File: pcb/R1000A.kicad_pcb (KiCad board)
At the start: 2 copper layers, 182 x 104 mm, 111 parts, among them J1 PCIESOCKET-X1, J10 PCIESOCKET-X1, J11 PCIESOCKET-X1, J12 PCIESOCKET-X1, J13 PCIESOCKET-X1, J14 PCIESOCKET-X1, J15 PCIESOCKET-X1, J16 PCIESOCKET-X1, J17 USB_B_RECEPTACLE, J18 USB_B_RECEPTACLE, J2 PCIESOCKET-X1, J25 SOCKET420P-02X04-CPU, J26 SOCKET508P-01X04, J27 CONN500P-01X04, J3 PCIESOCKET-X1, J4 PCIESOCKET-X1, J5 PCIESOCKET-X1, J6 PCIESOCKET-X1, J7 PCIESOCKET-X1, J8 PCIESOCKET-X1, J9 PCIESOCKET-X1, U1 LPC1769FBD100,551, U2 AP3418, U3 NX3DV221, U4 78SRH-5/2-C

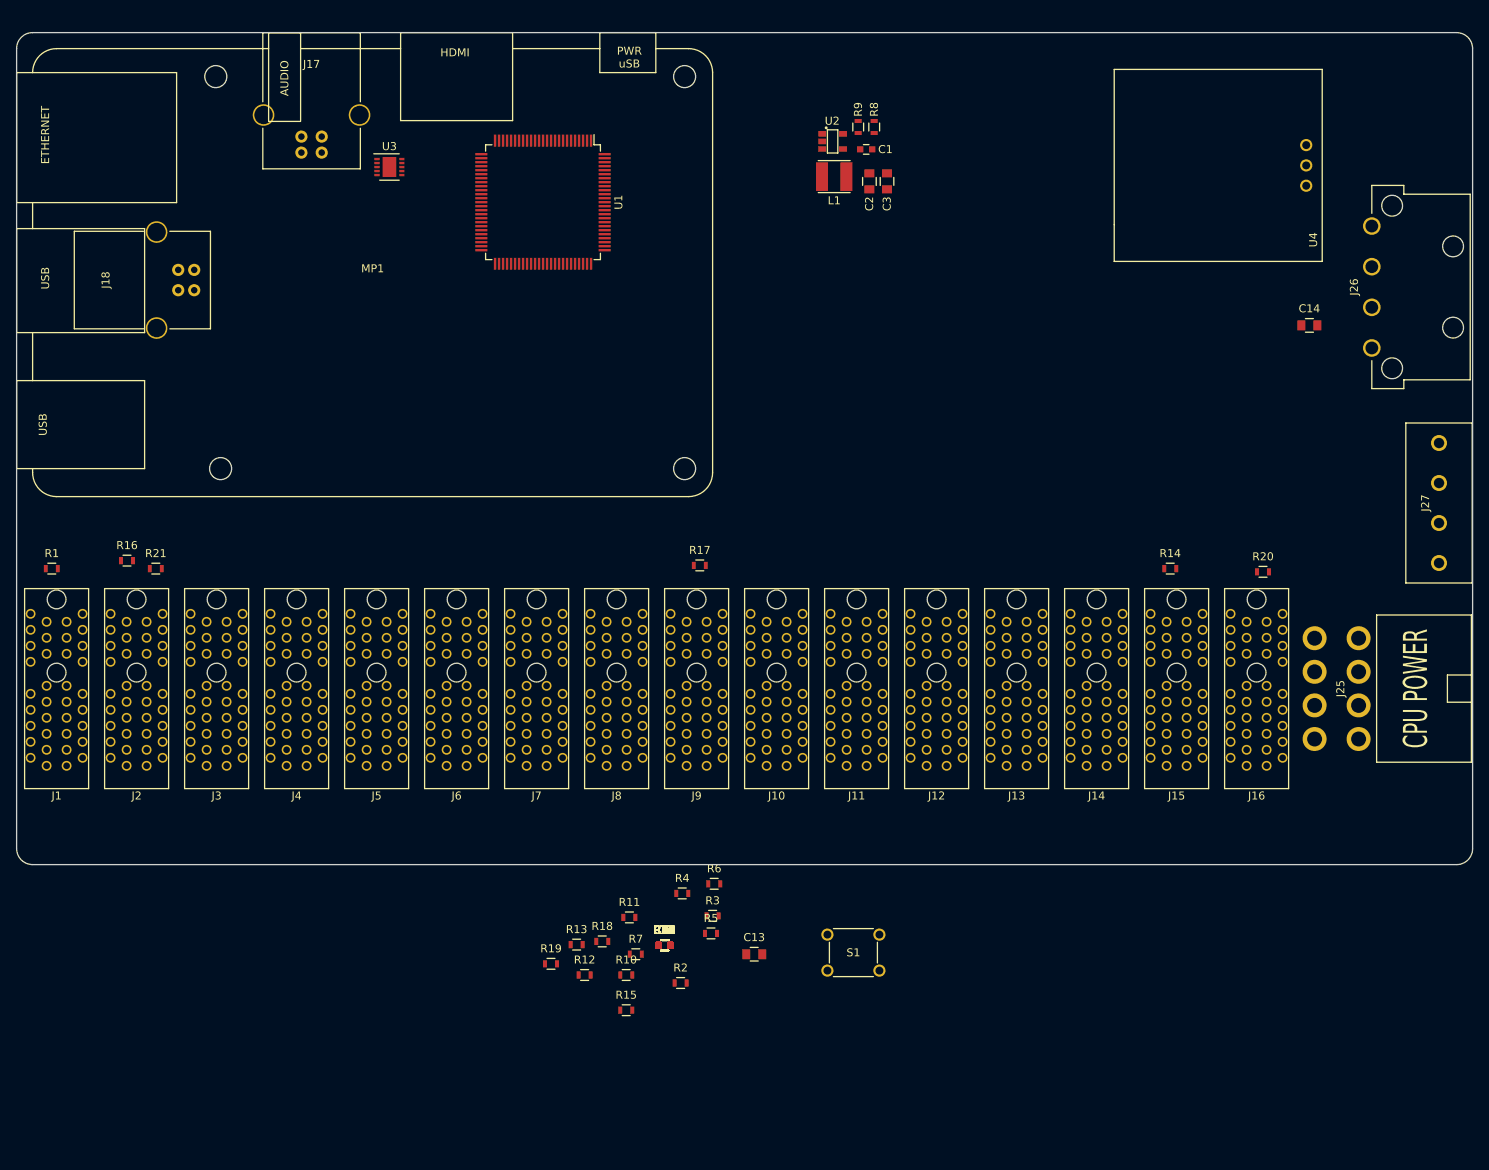
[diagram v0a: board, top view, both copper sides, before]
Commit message: layout wip
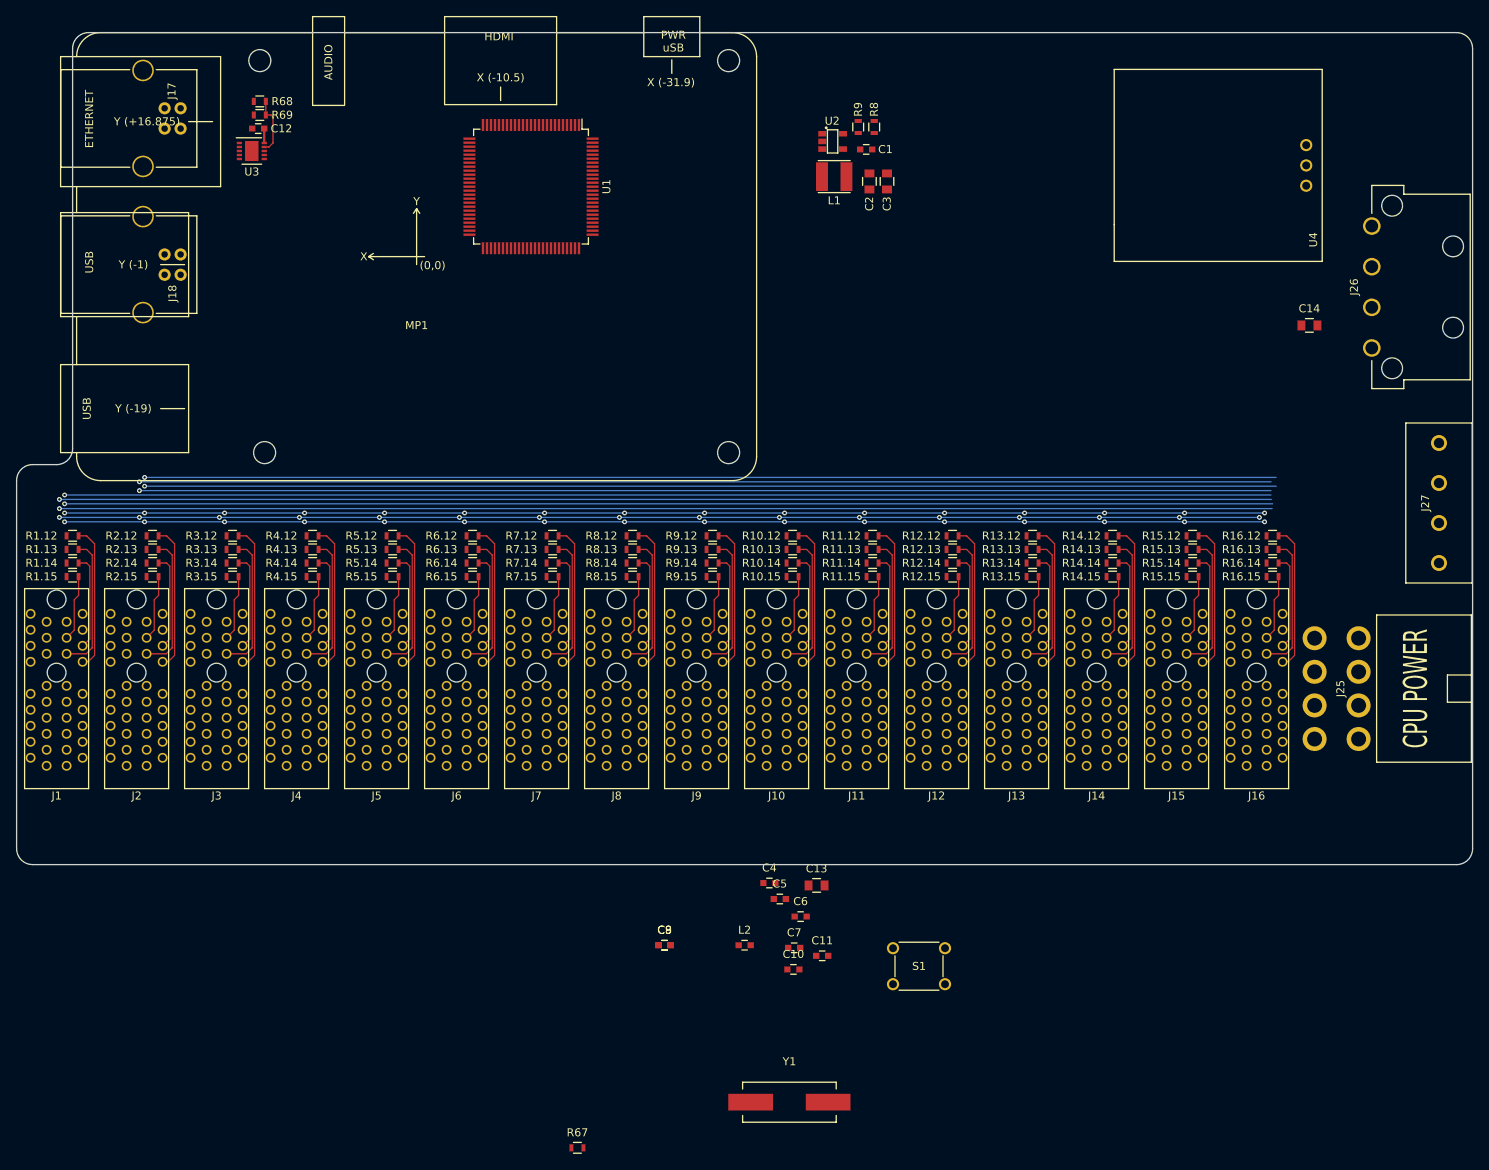
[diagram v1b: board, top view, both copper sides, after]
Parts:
- removed R1, R10, R11, R12, R13, R14, R15, R16, R17, R18, R19, R2, R20, R21, R22, R23, R24, R25, R26, R27, R28, R29, R3, R30, R31, R32, R33, R34, R35, R36, R37, R38, R39, R4, R40, R41, R42, R43, R44, R45, R46, R47, R48, R49, R5, R50, R51, R52, R53, R54, R55, R56, R57, R58, R59, R6, R60, R61, R62, R63, R64, R65, R66, R7: 10k, Resistors_SMD:R_0603
- added L2: 600Ohms, Capacitors_SMD:C_0603, F.Cu at (156.0, 152.1)
- added R1.12: 10k, Resistors_SMD:R_0603, F.Cu at (72.0, 100.9)
- added R1.13: 10k, Resistors_SMD:R_0603, F.Cu at (72.0, 102.6)
- added R1.14: 10k, Resistors_SMD:R_0603, F.Cu at (72.0, 104.3)
- added R1.15: 10k, Resistors_SMD:R_0603, F.Cu at (72.0, 106.0)
- added R10.12: 10k, Resistors_SMD:R_0603, F.Cu at (162.0, 100.9)
- added R10.13: 10k, Resistors_SMD:R_0603, F.Cu at (162.0, 102.6)
- added R10.14: 10k, Resistors_SMD:R_0603, F.Cu at (162.0, 104.3)
- added R10.15: 10k, Resistors_SMD:R_0603, F.Cu at (162.0, 106.0)
- added R11.12: 10k, Resistors_SMD:R_0603, F.Cu at (172.0, 100.9)
- added R11.13: 10k, Resistors_SMD:R_0603, F.Cu at (172.0, 102.6)
- added R11.14: 10k, Resistors_SMD:R_0603, F.Cu at (172.0, 104.3)
- added R11.15: 10k, Resistors_SMD:R_0603, F.Cu at (172.0, 106.0)
- added R12.12: 10k, Resistors_SMD:R_0603, F.Cu at (182.0, 100.9)
- added R12.13: 10k, Resistors_SMD:R_0603, F.Cu at (182.0, 102.6)
- added R12.14: 10k, Resistors_SMD:R_0603, F.Cu at (182.0, 104.3)
- added R12.15: 10k, Resistors_SMD:R_0603, F.Cu at (182.0, 106.0)
- added R13.12: 10k, Resistors_SMD:R_0603, F.Cu at (192.0, 100.9)
- added R13.13: 10k, Resistors_SMD:R_0603, F.Cu at (192.0, 102.6)
- added R13.14: 10k, Resistors_SMD:R_0603, F.Cu at (192.0, 104.3)
- added R13.15: 10k, Resistors_SMD:R_0603, F.Cu at (192.0, 106.0)
- added R14.12: 10k, Resistors_SMD:R_0603, F.Cu at (202.0, 100.9)
- added R14.13: 10k, Resistors_SMD:R_0603, F.Cu at (202.0, 102.6)
- added R14.14: 10k, Resistors_SMD:R_0603, F.Cu at (202.0, 104.3)
- added R14.15: 10k, Resistors_SMD:R_0603, F.Cu at (202.0, 106.0)
- added R15.12: 10k, Resistors_SMD:R_0603, F.Cu at (212.0, 100.9)
- added R15.13: 10k, Resistors_SMD:R_0603, F.Cu at (212.0, 102.6)
- added R15.14: 10k, Resistors_SMD:R_0603, F.Cu at (212.0, 104.3)
- added R15.15: 10k, Resistors_SMD:R_0603, F.Cu at (212.0, 106.0)
- added R16.12: 10k, Resistors_SMD:R_0603, F.Cu at (222.0, 100.9)
- added R16.13: 10k, Resistors_SMD:R_0603, F.Cu at (222.0, 102.6)
- added R16.14: 10k, Resistors_SMD:R_0603, F.Cu at (222.0, 104.3)
- added R16.15: 10k, Resistors_SMD:R_0603, F.Cu at (222.0, 106.0)
- added R2.12: 10k, Resistors_SMD:R_0603, F.Cu at (82.0, 100.9)
- added R2.13: 10k, Resistors_SMD:R_0603, F.Cu at (82.0, 102.6)
- added R2.14: 10k, Resistors_SMD:R_0603, F.Cu at (82.0, 104.3)
- added R2.15: 10k, Resistors_SMD:R_0603, F.Cu at (82.0, 106.0)
- added R3.12: 10k, Resistors_SMD:R_0603, F.Cu at (92.0, 100.9)
- added R3.13: 10k, Resistors_SMD:R_0603, F.Cu at (92.0, 102.6)
- added R3.14: 10k, Resistors_SMD:R_0603, F.Cu at (92.0, 104.3)
- added R3.15: 10k, Resistors_SMD:R_0603, F.Cu at (92.0, 106.0)
- added R4.12: 10k, Resistors_SMD:R_0603, F.Cu at (102.0, 100.9)
- added R4.13: 10k, Resistors_SMD:R_0603, F.Cu at (102.0, 102.6)
- added R4.14: 10k, Resistors_SMD:R_0603, F.Cu at (102.0, 104.3)
- added R4.15: 10k, Resistors_SMD:R_0603, F.Cu at (102.0, 106.0)
- added R5.12: 10k, Resistors_SMD:R_0603, F.Cu at (112.0, 100.9)
- added R5.13: 10k, Resistors_SMD:R_0603, F.Cu at (112.0, 102.6)
- added R5.14: 10k, Resistors_SMD:R_0603, F.Cu at (112.0, 104.3)
- added R5.15: 10k, Resistors_SMD:R_0603, F.Cu at (112.0, 106.0)
- added R6.12: 10k, Resistors_SMD:R_0603, F.Cu at (122.0, 100.9)
- added R6.13: 10k, Resistors_SMD:R_0603, F.Cu at (122.0, 102.6)
- added R6.14: 10k, Resistors_SMD:R_0603, F.Cu at (122.0, 104.3)
- added R6.15: 10k, Resistors_SMD:R_0603, F.Cu at (122.0, 106.0)
- added R7.12: 10k, Resistors_SMD:R_0603, F.Cu at (132.0, 100.9)
- added R7.13: 10k, Resistors_SMD:R_0603, F.Cu at (132.0, 102.6)
- added R7.14: 10k, Resistors_SMD:R_0603, F.Cu at (132.0, 104.3)
- added R7.15: 10k, Resistors_SMD:R_0603, F.Cu at (132.0, 106.0)
- added R8.12: 10k, Resistors_SMD:R_0603, F.Cu at (142.0, 100.9)
- added R8.13: 10k, Resistors_SMD:R_0603, F.Cu at (142.0, 102.6)
- added R8.14: 10k, Resistors_SMD:R_0603, F.Cu at (142.0, 104.3)
- added R8.15: 10k, Resistors_SMD:R_0603, F.Cu at (142.0, 106.0)
- added R9.12: 10k, Resistors_SMD:R_0603, F.Cu at (152.0, 100.9)
- added R9.13: 10k, Resistors_SMD:R_0603, F.Cu at (152.0, 102.6)
- added R9.14: 10k, Resistors_SMD:R_0603, F.Cu at (152.0, 104.3)
- added R9.15: 10k, Resistors_SMD:R_0603, F.Cu at (152.0, 106.0)
- added Y1: XTAL2_12MHz, Main:XTAL1140X470X420, F.Cu at (161.6, 171.7)
- MP1: footprint Main:DOCK_RPI -> Main:DOCK_RPI_Z020
- moved R68 117.0 mm to (95.4, 46.6)
- moved R69 115.5 mm to (95.4, 48.3), turned to 180 degrees
- moved C12 114.0 mm to (95.2, 50.0), turned to 180 degrees
- moved R67 27.6 mm to (135.1, 177.4)
- moved C11 19.7 mm to (165.7, 153.4)
- moved C6 17.4 mm to (163.0, 148.5)
- moved U3 17.3 mm to (94.4, 52.8)
- moved C10 16.4 mm to (162.1, 155.1)
- moved C7 16.2 mm to (162.2, 152.4)
- moved C5 15.5 mm to (160.4, 146.3)
- moved J17 15.4 mm to (85.5, 50.0), turned to 180 degrees
- moved C4 15.2 mm to (159.1, 144.3)
- moved C13 11.6 mm to (165.0, 144.6)
- moved S1 8.37 mm to (177.8, 154.7)
- moved MP1 5.85 mm to (115.0, 66.0)
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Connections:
- net Net-(J18-Pad1) renamed /VUSB_S
- J1 pad B12: Net-(J1-PadB12) -> /PCIeSockets/J1.B12
- J1 pad B13: Net-(J1-PadB13) -> /PCIeSockets/J1.B13
- J1 pad B14: Net-(J1-PadB14) -> /PCIeSockets/J1.B14
- J1 pad B15: Net-(J1-PadB15) -> /PCIeSockets/J1.B15
- J10 pad B12: Net-(J10-PadB12) -> /PCIeSockets/J10.B12
- J10 pad B13: Net-(J10-PadB13) -> /PCIeSockets/J10.B13
- J10 pad B14: Net-(J10-PadB14) -> /PCIeSockets/J10.B14
- J10 pad B15: Net-(J10-PadB15) -> /PCIeSockets/J10.B15
- J11 pad B12: Net-(J11-PadB12) -> /PCIeSockets/J11.B12
- J11 pad B13: Net-(J11-PadB13) -> /PCIeSockets/J11.B13
- J11 pad B14: Net-(J11-PadB14) -> /PCIeSockets/J11.B14
- J11 pad B15: Net-(J11-PadB15) -> /PCIeSockets/J11.B15
- J12 pad B12: Net-(J12-PadB12) -> /PCIeSockets/J12.B12
- J12 pad B13: Net-(J12-PadB13) -> /PCIeSockets/J12.B13
- J12 pad B14: Net-(J12-PadB14) -> /PCIeSockets/J12.B14
- J12 pad B15: Net-(J12-PadB15) -> /PCIeSockets/J12.B15
- J13 pad B12: Net-(J13-PadB12) -> /PCIeSockets/J13.B12
- J13 pad B13: Net-(J13-PadB13) -> /PCIeSockets/J13.B13
- J13 pad B14: Net-(J13-PadB14) -> /PCIeSockets/J13.B14
- J13 pad B15: Net-(J13-PadB15) -> /PCIeSockets/J13.B15
- J14 pad B12: Net-(J14-PadB12) -> /PCIeSockets/J14.B12
- J14 pad B13: Net-(J14-PadB13) -> /PCIeSockets/J14.B13
- J14 pad B14: Net-(J14-PadB14) -> /PCIeSockets/J14.B14
- J14 pad B15: Net-(J14-PadB15) -> /PCIeSockets/J14.B15
- J15 pad B12: Net-(J15-PadB12) -> /PCIeSockets/J15.B12
- J15 pad B13: Net-(J15-PadB13) -> /PCIeSockets/J15.B13
- J15 pad B14: Net-(J15-PadB14) -> /PCIeSockets/J15.B14
- J15 pad B15: Net-(J15-PadB15) -> /PCIeSockets/J15.B15
- J16 pad B12: Net-(J16-PadB12) -> /PCIeSockets/J16.B12
- J16 pad B13: Net-(J16-PadB13) -> /PCIeSockets/J16.B13
- J16 pad B14: Net-(J16-PadB14) -> /PCIeSockets/J16.B14
- J16 pad B15: Net-(J16-PadB15) -> /PCIeSockets/J16.B15
- J2 pad B12: Net-(J2-PadB12) -> /PCIeSockets/J2.B12
- J2 pad B13: Net-(J2-PadB13) -> /PCIeSockets/J2.B13
- J2 pad B14: Net-(J2-PadB14) -> /PCIeSockets/J2.B14
- J2 pad B15: Net-(J2-PadB15) -> /PCIeSockets/J2.B15
- J3 pad B12: Net-(J3-PadB12) -> /PCIeSockets/J3.B12
- J3 pad B13: Net-(J3-PadB13) -> /PCIeSockets/J3.B13
- J3 pad B14: Net-(J3-PadB14) -> /PCIeSockets/J3.B14
- J3 pad B15: Net-(J3-PadB15) -> /PCIeSockets/J3.B15
- J4 pad B12: Net-(J4-PadB12) -> /PCIeSockets/J4.B12
- J4 pad B13: Net-(J4-PadB13) -> /PCIeSockets/J4.B13
- J4 pad B14: Net-(J4-PadB14) -> /PCIeSockets/J4.B14
- J4 pad B15: Net-(J4-PadB15) -> /PCIeSockets/J4.B15
- J5 pad B12: Net-(J5-PadB12) -> /PCIeSockets/J5.B12
- J5 pad B13: Net-(J5-PadB13) -> /PCIeSockets/J5.B13
- J5 pad B14: Net-(J5-PadB14) -> /PCIeSockets/J5.B14
- J5 pad B15: Net-(J5-PadB15) -> /PCIeSockets/J5.B15
- J6 pad B12: Net-(J6-PadB12) -> /PCIeSockets/J6.B12
- J6 pad B13: Net-(J6-PadB13) -> /PCIeSockets/J6.B13
- J6 pad B14: Net-(J6-PadB14) -> /PCIeSockets/J6.B14
- J6 pad B15: Net-(J6-PadB15) -> /PCIeSockets/J6.B15
- J7 pad B12: Net-(J7-PadB12) -> /PCIeSockets/J7.B12
- J7 pad B13: Net-(J7-PadB13) -> /PCIeSockets/J7.B13
- J7 pad B14: Net-(J7-PadB14) -> /PCIeSockets/J7.B14
- J7 pad B15: Net-(J7-PadB15) -> /PCIeSockets/J7.B15
- J8 pad B12: Net-(J8-PadB12) -> /PCIeSockets/J8.B12
- J8 pad B13: Net-(J8-PadB13) -> /PCIeSockets/J8.B13
- J8 pad B14: Net-(J8-PadB14) -> /PCIeSockets/J8.B14
- J8 pad B15: Net-(J8-PadB15) -> /PCIeSockets/J8.B15
- J9 pad B12: Net-(J9-PadB12) -> /PCIeSockets/J9.B12
- J9 pad B13: Net-(J9-PadB13) -> /PCIeSockets/J9.B13
- J9 pad B14: Net-(J9-PadB14) -> /PCIeSockets/J9.B14
- J9 pad B15: Net-(J9-PadB15) -> /PCIeSockets/J9.B15
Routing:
- net (no net): track 0.00 -> 604.9 mm, vias 0 -> 4
- net SCL0: track 0.00 -> 460.4 mm, vias 0 -> 16
- net SDA0: track 0.00 -> 414.4 mm, vias 0 -> 16
- net ~MRESET: track 0.00 -> 407.7 mm, vias 0 -> 16
- net J02.PX1.A12: track 0.00 -> 171.5 mm, vias 0 -> 1
- net J02.PX2.A13: track 0.00 -> 169.8 mm, vias 0 -> 1
- net J02.PX3.A14: track 0.00 -> 166.9 mm, vias 0 -> 1
- net J02.PX4.A15: track 0.00 -> 163.2 mm, vias 0 -> 1
- net J16.PX1.A12: track 0.00 -> 23.7 mm
- net J15.PX1.A12: track 0.00 -> 23.7 mm
- net J14.PX1.A12: track 0.00 -> 23.7 mm
- net J13.PX1.A12: track 0.00 -> 23.7 mm
- net J12.PX1.A12: track 0.00 -> 23.7 mm
- net J11.PX1.A12: track 0.00 -> 23.7 mm
- net J10.PX1.A12: track 0.00 -> 23.7 mm
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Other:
- outline, holes or cut-outs redrawn
- copper layers 2 -> 4
